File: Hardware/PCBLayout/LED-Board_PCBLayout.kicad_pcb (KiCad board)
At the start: 2 copper layers, 100 x 100 mm, 11 parts, among them U1 L78L05_TO92

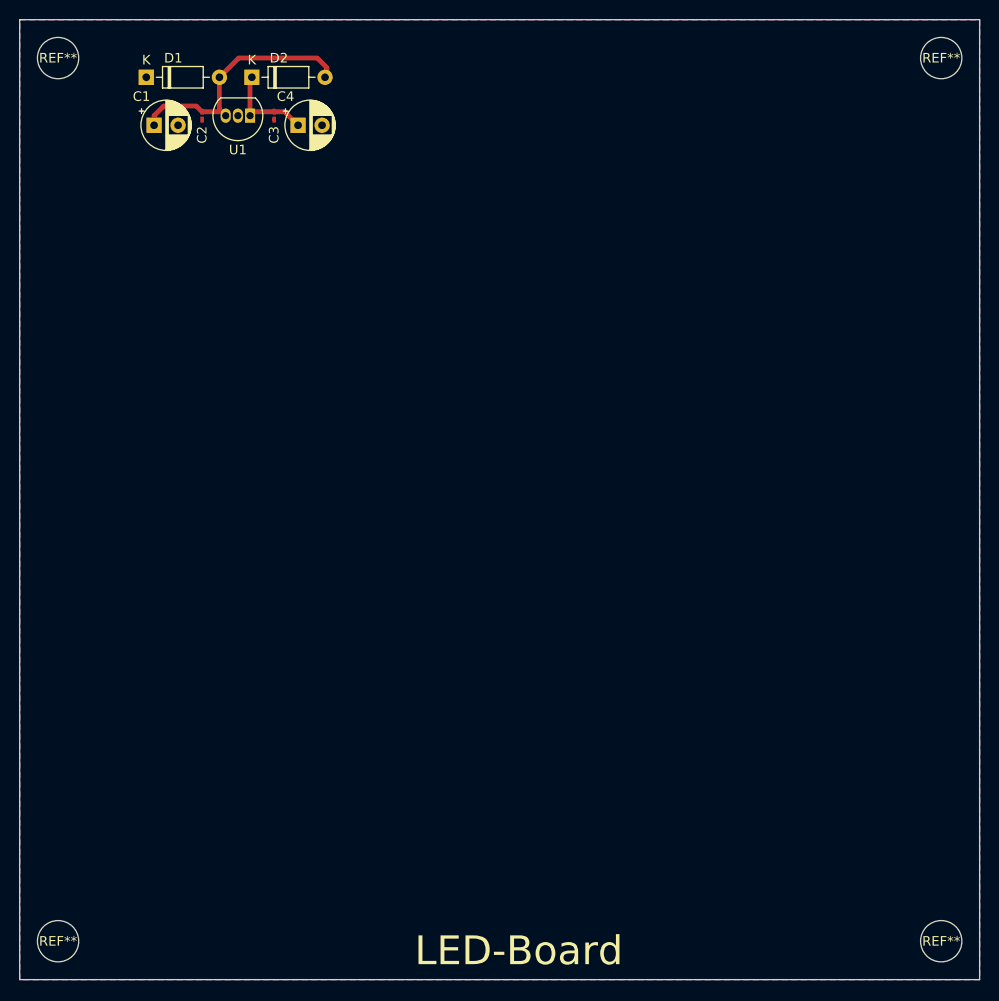
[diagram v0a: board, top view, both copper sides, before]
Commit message: power supply / power unit
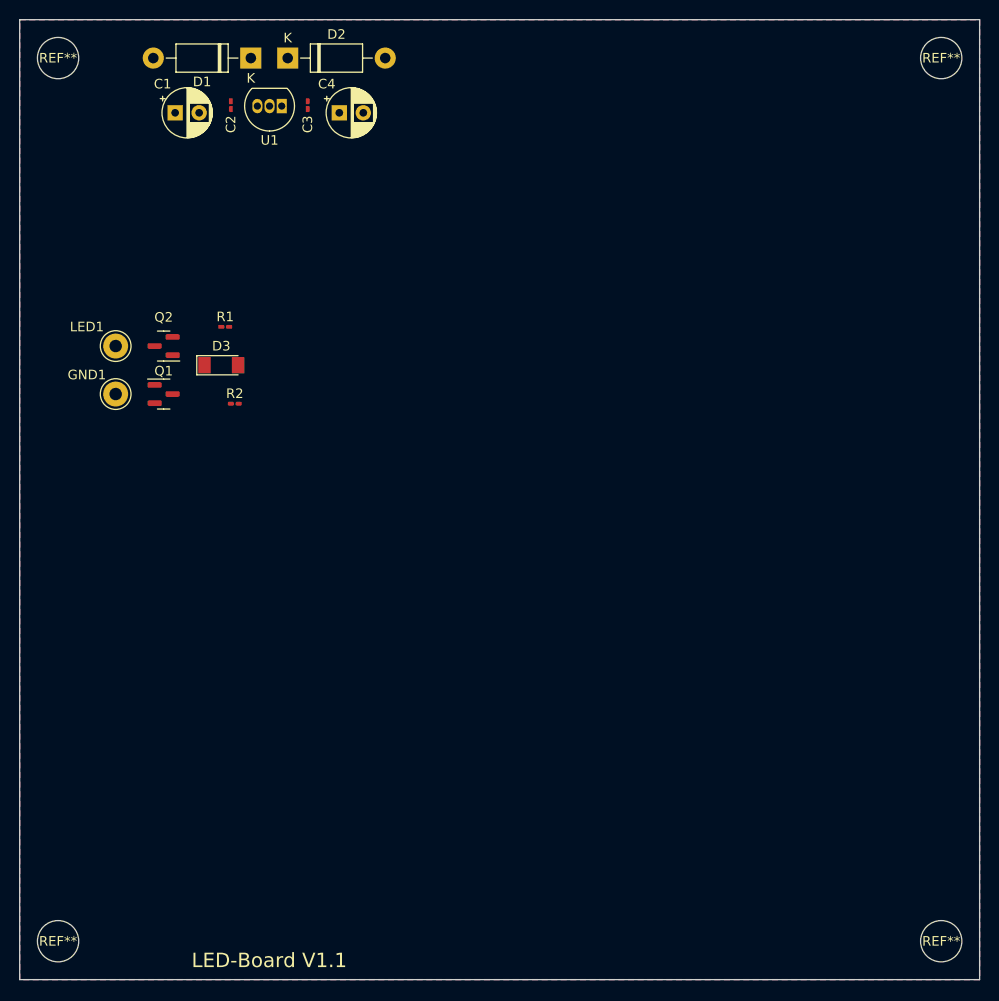
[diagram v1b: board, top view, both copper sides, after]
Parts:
- added  : Layer1, Pabst:Layer1, F.Cu at (32.0, 117.0)
- added  : Layer2, Pabst:Layer2, F.Cu at (32.0, 117.0)
- added D3: BZV55C3V3, Diode_SMD:D_MiniMELF, F.Cu at (41.0, 56.0)
- added GND1: MHole, Connector_Pin:Pin_D1.3mm_L11.0mm, F.Cu at (30.0, 59.0)
- added LED1: MHole, Connector_Pin:Pin_D1.3mm_L11.0mm, F.Cu at (30.0, 54.0)
- added Q1: BC846, Package_TO_SOT_SMD:SOT-23, F.Cu at (35.0, 59.0)
- added Q2: BC856, Package_TO_SOT_SMD:SOT-23, F.Cu at (35.0, 54.0)
- added R1: R_Small, Resistor_SMD:R_0201_0603Metric_Pad0.64x0.40mm_HandSolder, F.Cu at (41.4, 52.0)
- added R2: R_Small, Resistor_SMD:R_0201_0603Metric_Pad0.64x0.40mm_HandSolder, F.Cu at (42.4, 60.0)
- D1, D2: value DIODE -> 1N4006; footprint Diode_THT:D_DO-35_SOD27_P7.62mm_Horizontal -> Diode_THT:D_DO-41_SOD81_P10.16mm_Horizontal
- moved D1 11.1 mm to (44.1, 24.0), turned to 180 degrees
- moved C4 4.49 mm to (53.3, 29.7)
- moved D2 4.23 mm to (47.9, 24.0)
- moved C3 3.67 mm to (50.0, 28.9)
- moved U1 3.45 mm to (47.3, 29.0)
- moved C2 3.20 mm to (42.0, 28.9)
- moved C1 2.55 mm to (36.2, 29.7)
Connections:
- C1 pad 1: Net-(C1-Pad1) -> +12V
- C2 pad 1: Net-(C1-Pad1) -> +12V
- D1 pad 2: Net-(C1-Pad1) -> +12V
- D2 pad 1: Net-(C3-Pad1) -> +12V
- D2 pad 2: Net-(C1-Pad1) -> Net-(C3-Pad1)
- U1 pad 3: Net-(C1-Pad1) -> +12V
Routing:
- net Net-(C1-Pad1): track 27.3 -> 0.00 mm
- net Net-(C3-Pad1): track 10.1 -> 0.00 mm
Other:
- board text added: "LED-Board V1.1"
- board text removed: "LED-Board"
